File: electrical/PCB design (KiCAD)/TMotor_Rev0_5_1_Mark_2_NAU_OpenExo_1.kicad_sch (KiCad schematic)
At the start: 10 parts, among them J1 Conn_01x07_Pin, U1 TXU0104PWR, U10 DEV-16771, U2 TXU0304-Q1

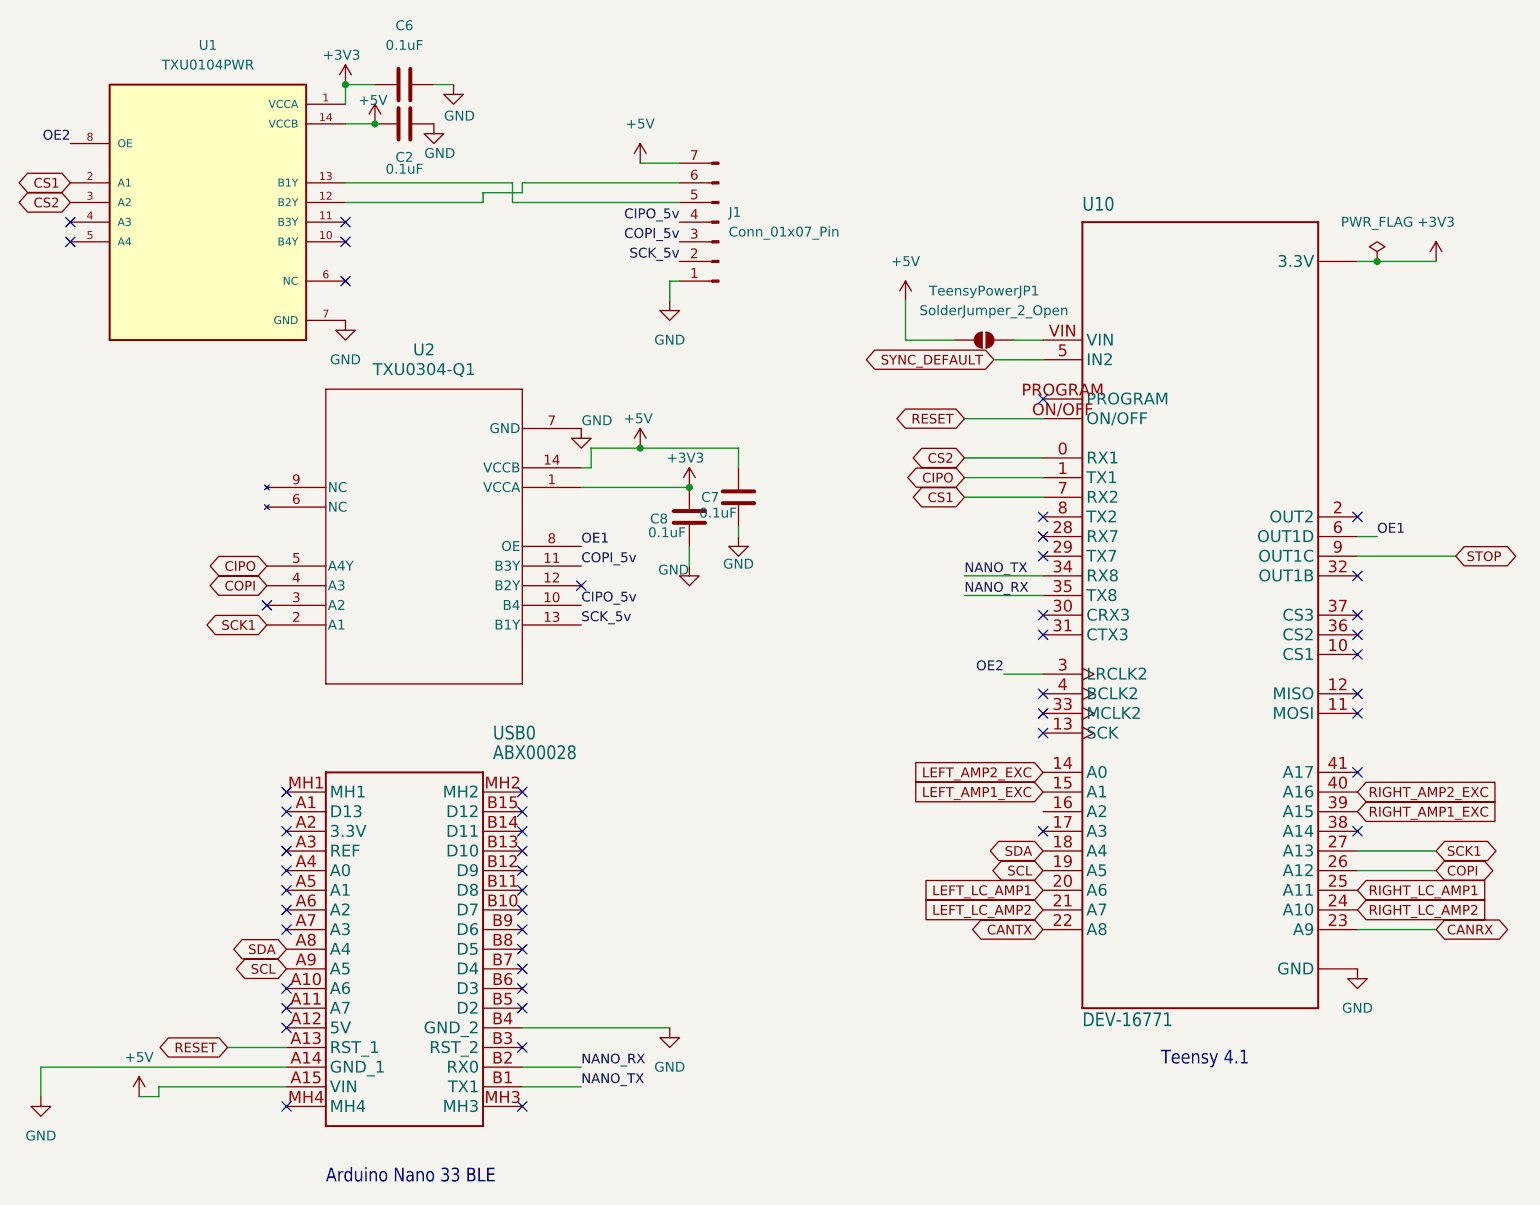
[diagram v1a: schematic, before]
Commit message: PCB version v1.1.0 design+documentation
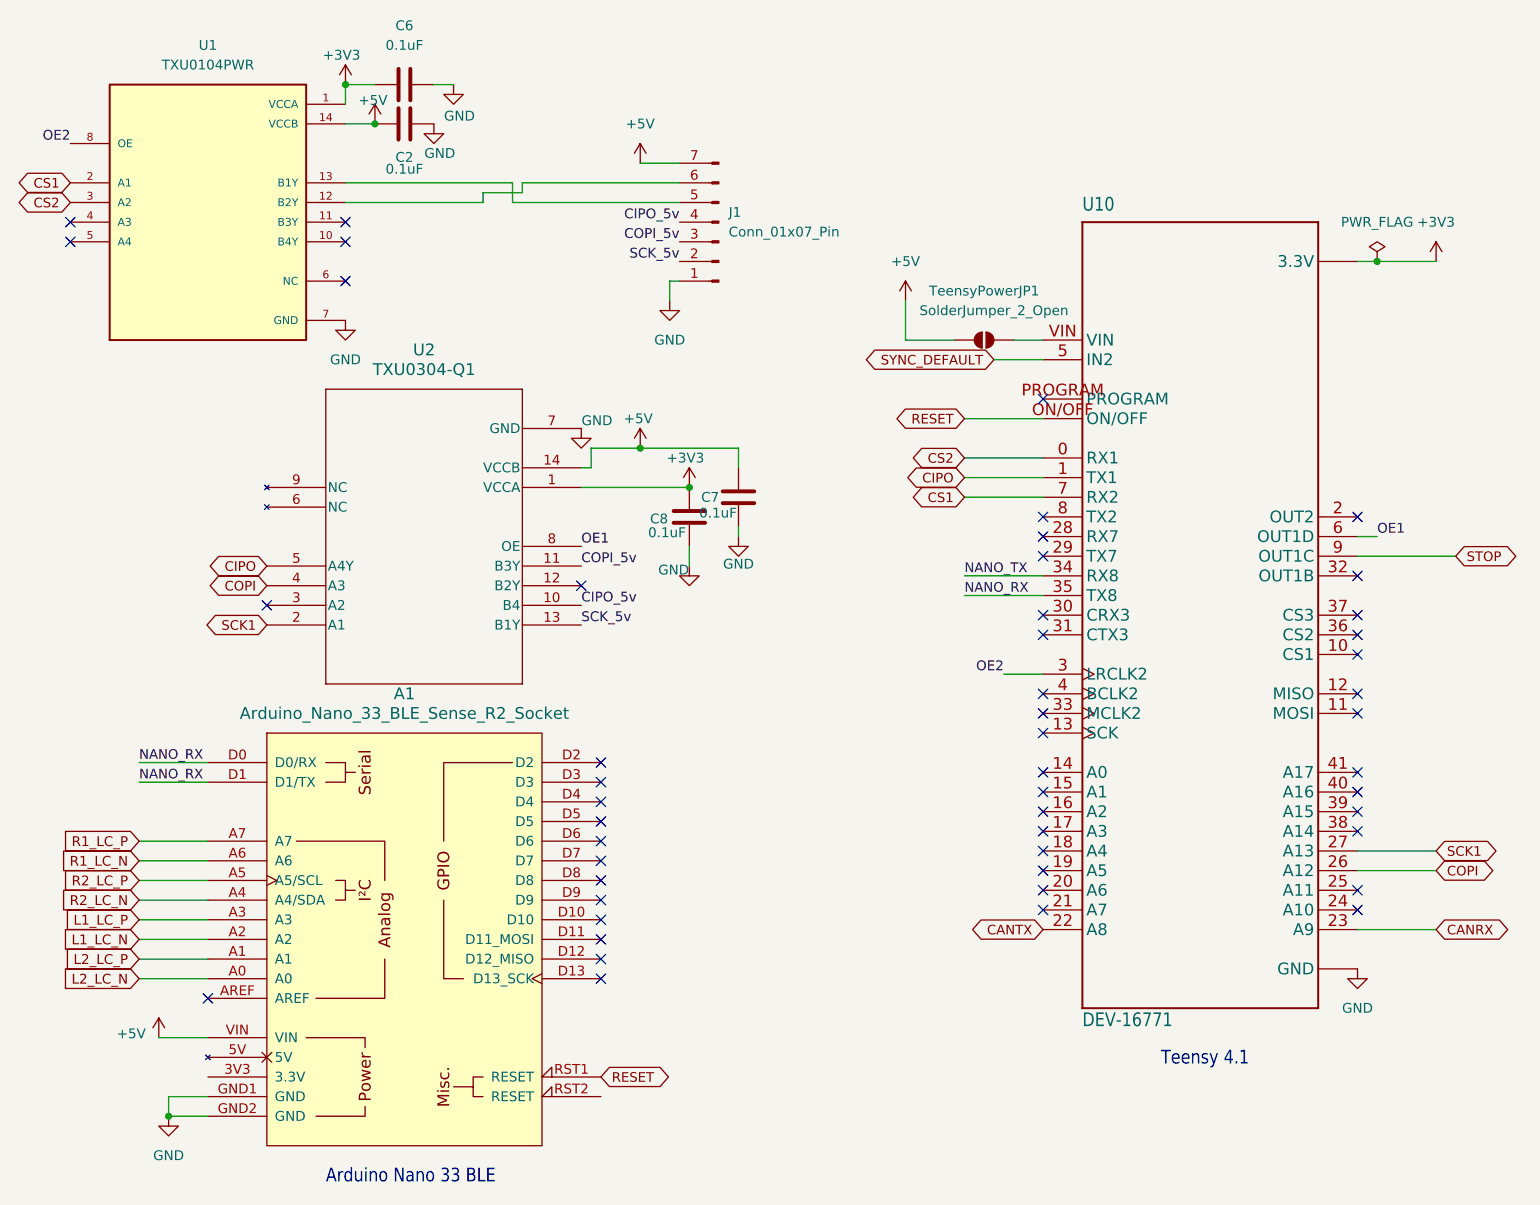
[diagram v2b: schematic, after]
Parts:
- removed USB0: ABX00028, TMotor_Rev0_5_1_Mark_2_NAU_OpenExo:ABX00028, symbol TMotor_Rev0_5_1_Mark_2_NAU_OpenExo-eagle-import:ABX00028
- added A1: Arduino_Nano_33_BLE_Sense_R2_Socket, PCM_arduino-library:Arduino_Nano_Every_Socket, symbol PCM_arduino-library:Arduino_Nano_33_BLE_Sense_R2_Socket
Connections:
- net +5V: now also A1.VIN
- net GND: now also A1.GND1 (GND), A1.GND2 (GND)
- net NANO_RX: now also A1.D0 (D0/RX), A1.D1 (D1/TX)
- net RESET: now also A1.RST1 (RESET)
- net LEFT_AMP1_EXC: no longer names the net of U10.15 (A1)
- net LEFT_AMP2_EXC: no longer names the net of U10.14 (A0)
- net LEFT_LC_AMP1: no longer names the net of U10.20 (A6)
- net LEFT_LC_AMP2: no longer names the net of U10.21 (A7)
- net RIGHT_AMP1_EXC: no longer names the net of U10.39 (A15)
- net RIGHT_AMP2_EXC: no longer names the net of U10.40 (A16)
- net RIGHT_LC_AMP1: no longer names the net of U10.25 (A11)
- net RIGHT_LC_AMP2: no longer names the net of U10.24 (A10)
- net SCL: no longer names the net of U10.19 (A5)
- net SDA: no longer names the net of U10.18 (A4)
- new net L1_LC_N: A1.A2
- new net L1_LC_P: A1.A3
- new net L2_LC_N: A1.A0
- new net L2_LC_P: A1.A1
- new net R1_LC_N: A1.A6
- new net R1_LC_P: A1.A7
- new net R2_LC_N: A1.A4 (A4/SDA)
- new net R2_LC_P: A1.A5 (A5/SCL)
- no-connect marks 52 -> 50
